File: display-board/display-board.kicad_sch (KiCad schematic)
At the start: 8 parts, among them J1 TO_PWR_BOARD, J2 OLED DISPLAY, SW1 X, SW2 BUTTON_DOWN, SW3 BUTTON_UP, SW4 BUTTON_TIME

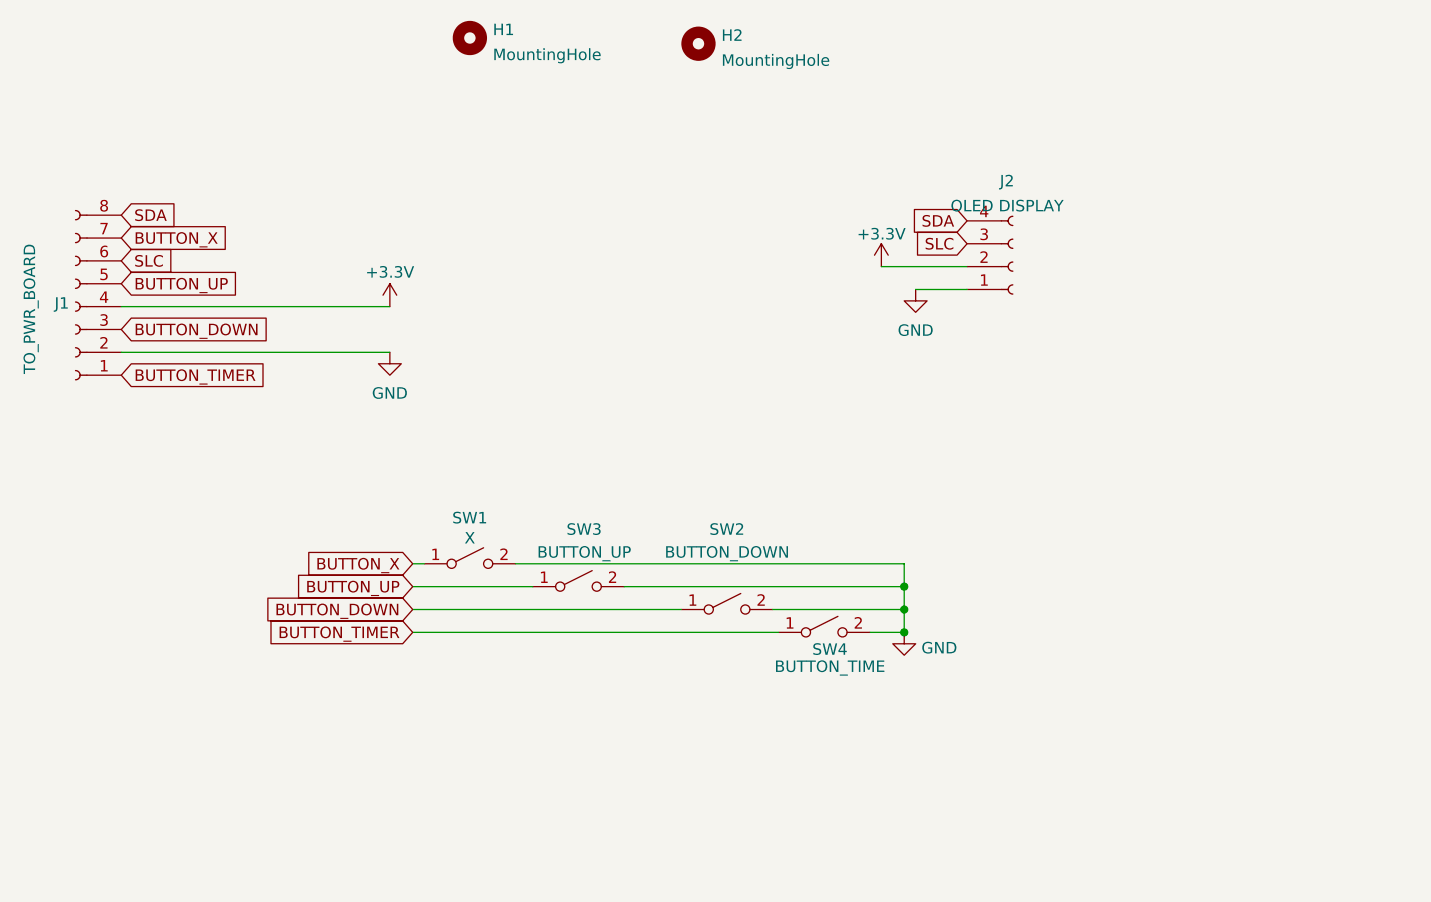
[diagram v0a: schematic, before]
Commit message: documentation
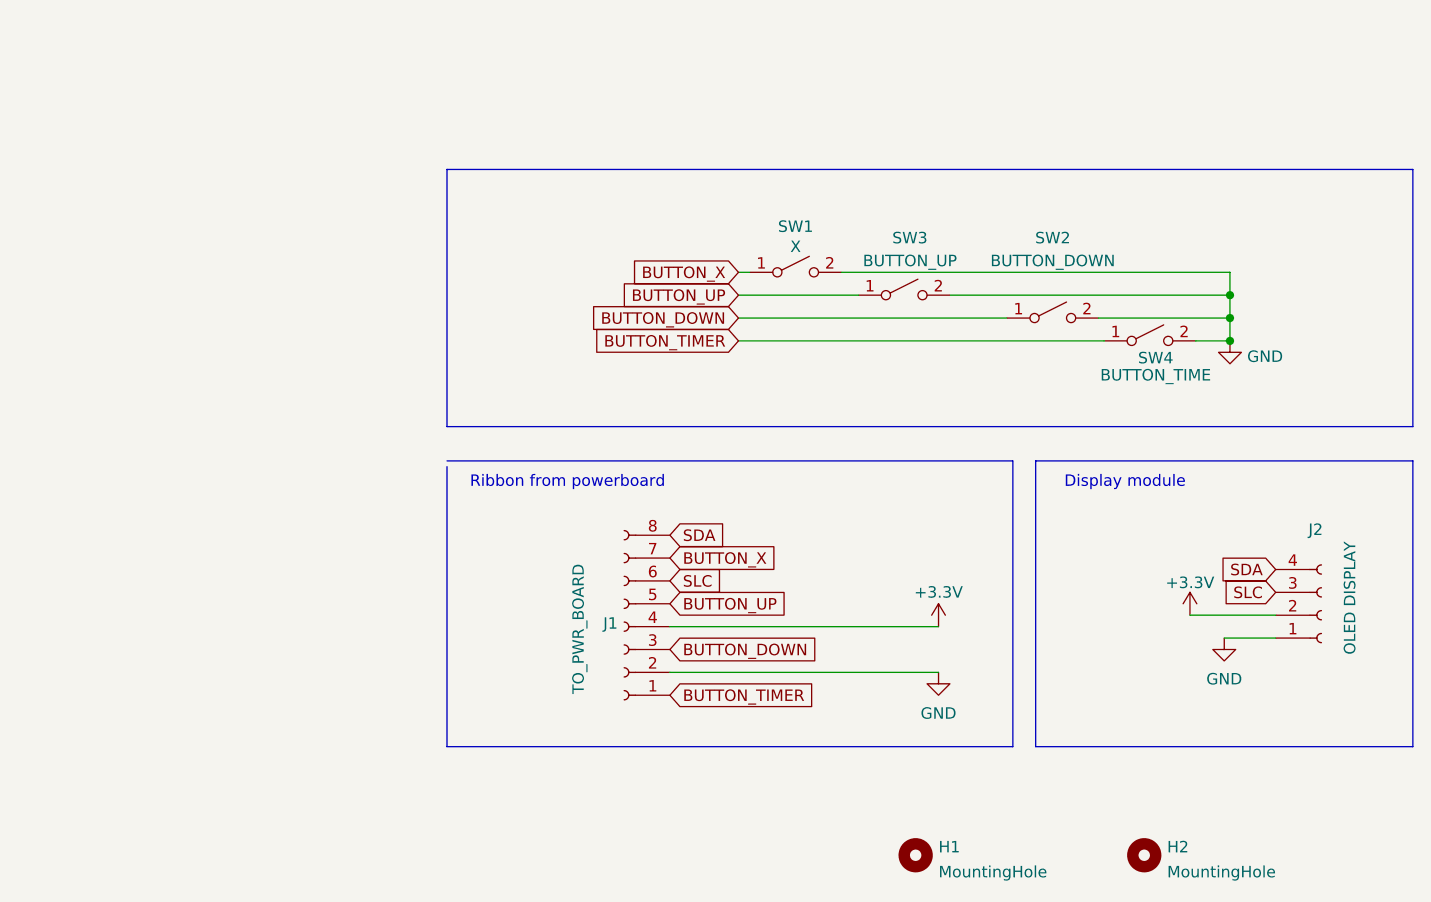
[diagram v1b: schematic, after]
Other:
- note added: "Display module"
- note added: "Ribbon from powerboard"
- moved on the sheet: H1, H2, J1, J2, SW1, SW2, SW3, SW4
